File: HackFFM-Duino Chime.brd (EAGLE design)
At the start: 15.2 x 30.5 mm, 63 parts, among them IC1 ATMEGA328, IC2 SN74LVC2G14, IC3 74LVC1G53DP, Q1 16MHz, U2 3.3V MIC5205, U3 MAX98306ETD+, U4 3.3V MIC5205

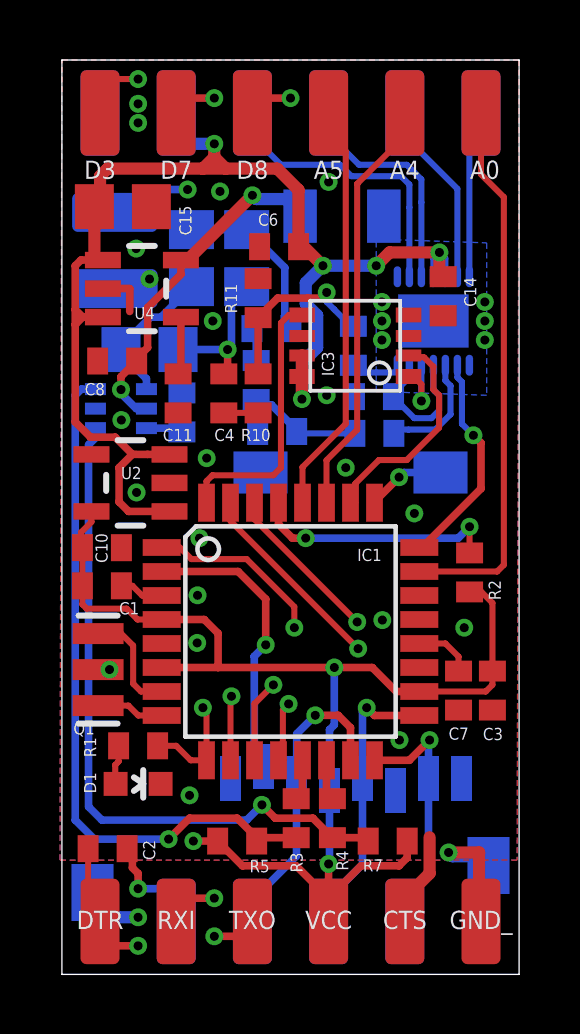
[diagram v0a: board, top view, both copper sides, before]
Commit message: Version 1.1 update
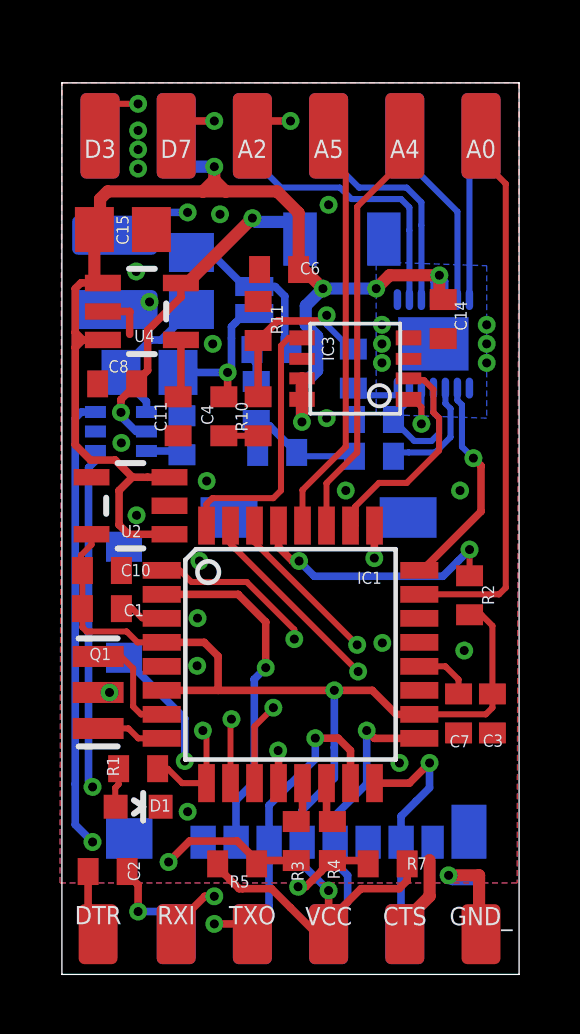
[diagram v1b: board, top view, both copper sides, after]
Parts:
- removed D8: M01M01_SMDSHORT_NOCREAM, MyEagleLibrary:M01_SMDSHORT_NOCREAM
- removed MONO_R0: 0R, MyEagleLibrary:R0805_NOCREAM
- removed U$1: MICROSD, MyEagleLibrary:MICROSD
- added A2: M01M01_SMD_EDGE_SHORT, MyEagleLibrary:M01_SMD_EDGE_SHORT
- added SJ1: SOLDERJUMPERNO, SparkFun:SJ_2S-NO
- added XU1: MICROSD_DETMOLEX104031, DCEM-microSD:MICROSD_MOLEX_104031
- +5V, 1+, 1-, 2+, 2-, A0, A4, A5, D3, D5, D6, D7, GND: value M01M01_SMDSHORT_NOCREAM -> M01M01_SMD_EDGE_SHORT; device MyEagleLibrary:M01_SMDSHORT_NOCREAM -> MyEagleLibrary:M01_SMD_EDGE_SHORT
- CTS, DTR, GND_, MISO, MOSI, RST, RXI, SCK, TXO, VCC: value M01M01_SMDSHORT_NOCREAM -> M01M01_SMD_EDGE_XS; device MyEagleLibrary:M01_SMDSHORT_NOCREAM -> MyEagleLibrary:M01_SMD_EDGE_XS
- moved +5V 1.84 mm to (3.81, 28.4)
- moved 1+ 1.84 mm to (11.4, 28.4)
- moved 1- 1.84 mm to (14.0, 28.4)
- moved 2+ 1.84 mm to (8.89, 28.4)
- moved 2- 1.84 mm to (6.35, 28.4)
- moved A0 1.84 mm to (14.0, 28.4)
- moved A4 1.84 mm to (11.4, 28.4)
- moved A5 1.84 mm to (8.89, 28.4)
- moved D3 1.84 mm to (1.27, 28.4)
- moved D7 1.84 mm to (3.81, 28.4)
- moved GND 1.84 mm to (1.27, 28.4)
- moved D6 1.32 mm to (1.27, 24.6)
- moved D5 1.29 mm to (1.27, 22.2)
- moved DTR 1.08 mm to (1.21, 1.27)
- moved CTS 1.08 mm to (11.4, 1.27)
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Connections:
- removed net 3.3V: C1.1, C10.1, C3.2, IC1.18, IC1.4, IC1.6, R2.2, R5.2, R7.2, U$1.4, U2.5, VCC.P$1
- new net +3V3: C1.1, C10.1, C3.2, IC1.18, IC1.4, IC1.6, R2.2, R5.2, R7.2, U2.5, VCC.P$1, XU1.4
- net A2: now also A2.P$1; no longer U$1.CD1
- net D4: now also XU1.2; no longer U$1.2
- net D8: now also XU1.DET_A; no longer D8.P$1
- net GND: now also XU1.6, XU1.DET_B, XU1.G1, XU1.G2, XU1.G3, XU1.G4; no longer U$1.6, U$1.CD2, U$1.MT1, U$1.MT2
- net MISO: now also XU1.7; no longer U$1.7
- net MOSI: now also XU1.3; no longer U$1.3
- net N$15: now also SJ1.1; no longer MONO_R0.1
- net N$17: now also SJ1.2; no longer MONO_R0.2
- net SCK: now also XU1.5; no longer U$1.5
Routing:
- net 3.3V: track 42.5 -> 0.00 mm, vias 3 -> 0
- net +3V3: track 0.00 -> 42.3 mm, vias 0 -> 2
- net D8: track 26.4 -> 8.63 mm
- net A2: track 2.64 -> 18.6 mm, vias 1 -> 2
- net N$5: track 23.0 -> 26.9 mm, vias 1 -> 2
- net DTR: track 5.36 -> 2.42 mm, vias 1 -> 0
- net GND: track 13.5 -> 11.1 mm
- net D4: track 9.72 -> 11.6 mm
- net TXO: track 20.6 -> 19.5 mm
- net D5: track 20.9 -> 19.9 mm
- net RST: track 37.0 -> 36.1 mm
- net D3: track 29.6 -> 28.7 mm
- net RXI: track 19.0 -> 18.2 mm
- net N$8: track 23.2 -> 22.9 mm, vias 1 -> 2
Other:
- board size 15.2 x 30.5 mm -> 15.2 x 29.7 mm
- board text removed: "Merges"
